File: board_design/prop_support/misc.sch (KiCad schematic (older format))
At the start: 14 parts

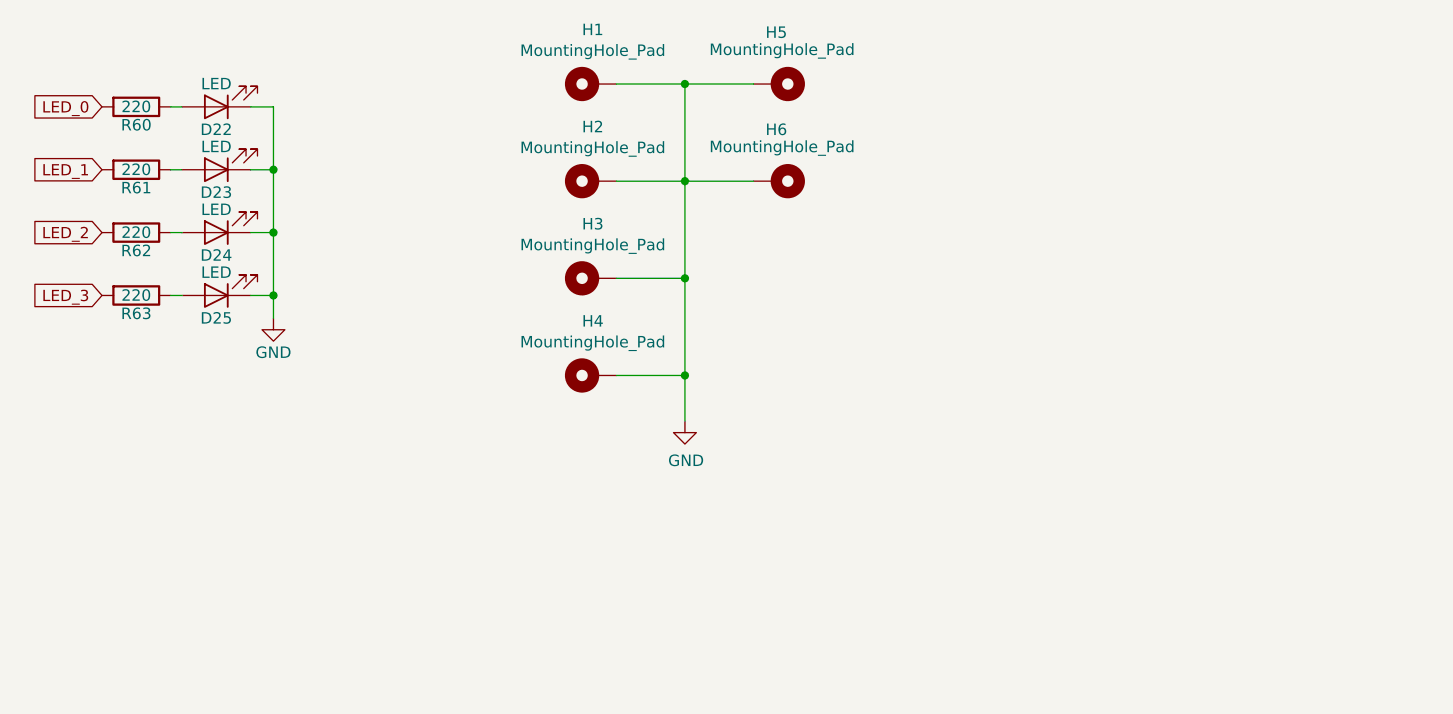
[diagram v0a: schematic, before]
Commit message: first MX export
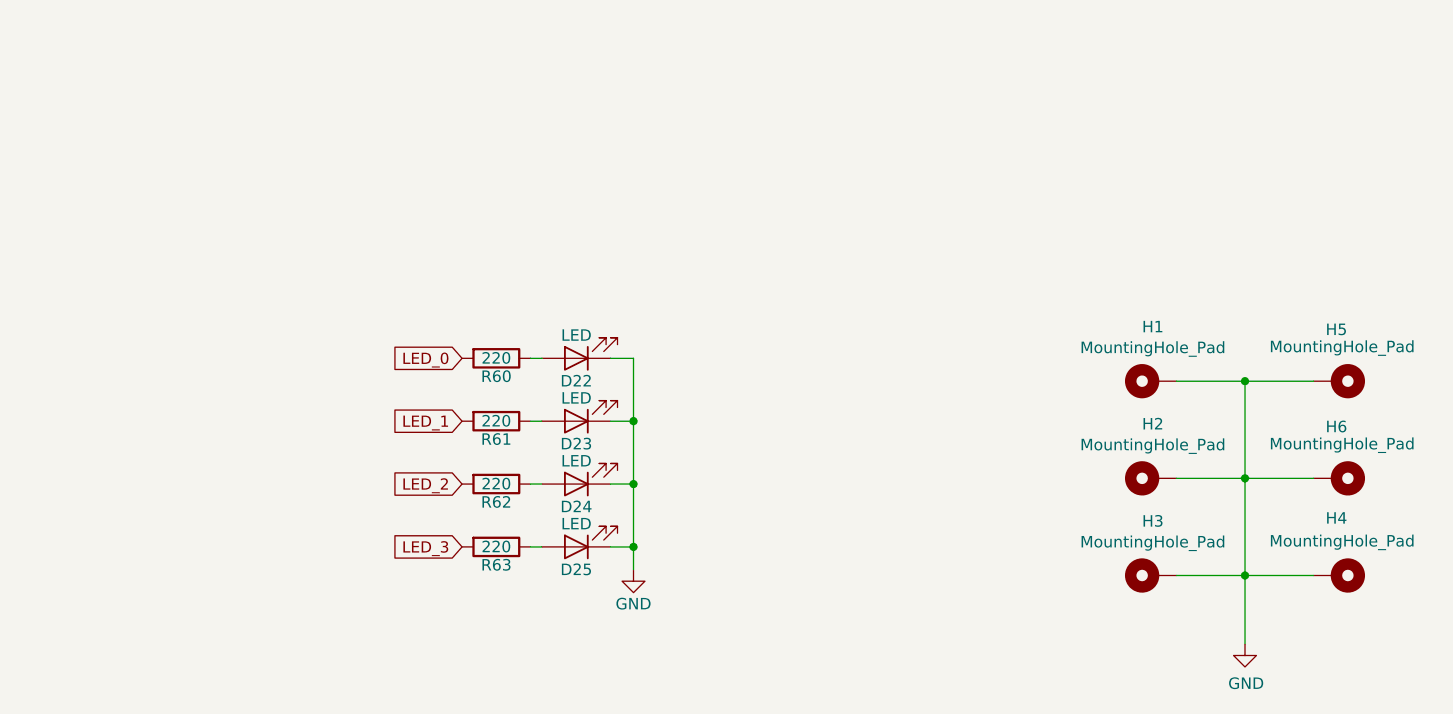
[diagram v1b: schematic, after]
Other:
- moved on the sheet: D22, D23, D24, D25, H1, H2, H3, H4, H5, H6, R60, R61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
